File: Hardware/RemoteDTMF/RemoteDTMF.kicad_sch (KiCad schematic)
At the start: 35 parts, among them J1 REG. 7V, J10 MT8870D, J11 P12V, J2 BATT 12V, J3 P12V, J4 Analog, J5 Digital, J6 TRX TELCO, J7 AL. ATTINY85, J8 IO ATTINY85, J9 AT-D578, U1 PC817, U2 PC817, U3 CD4066BE, U4 PC817

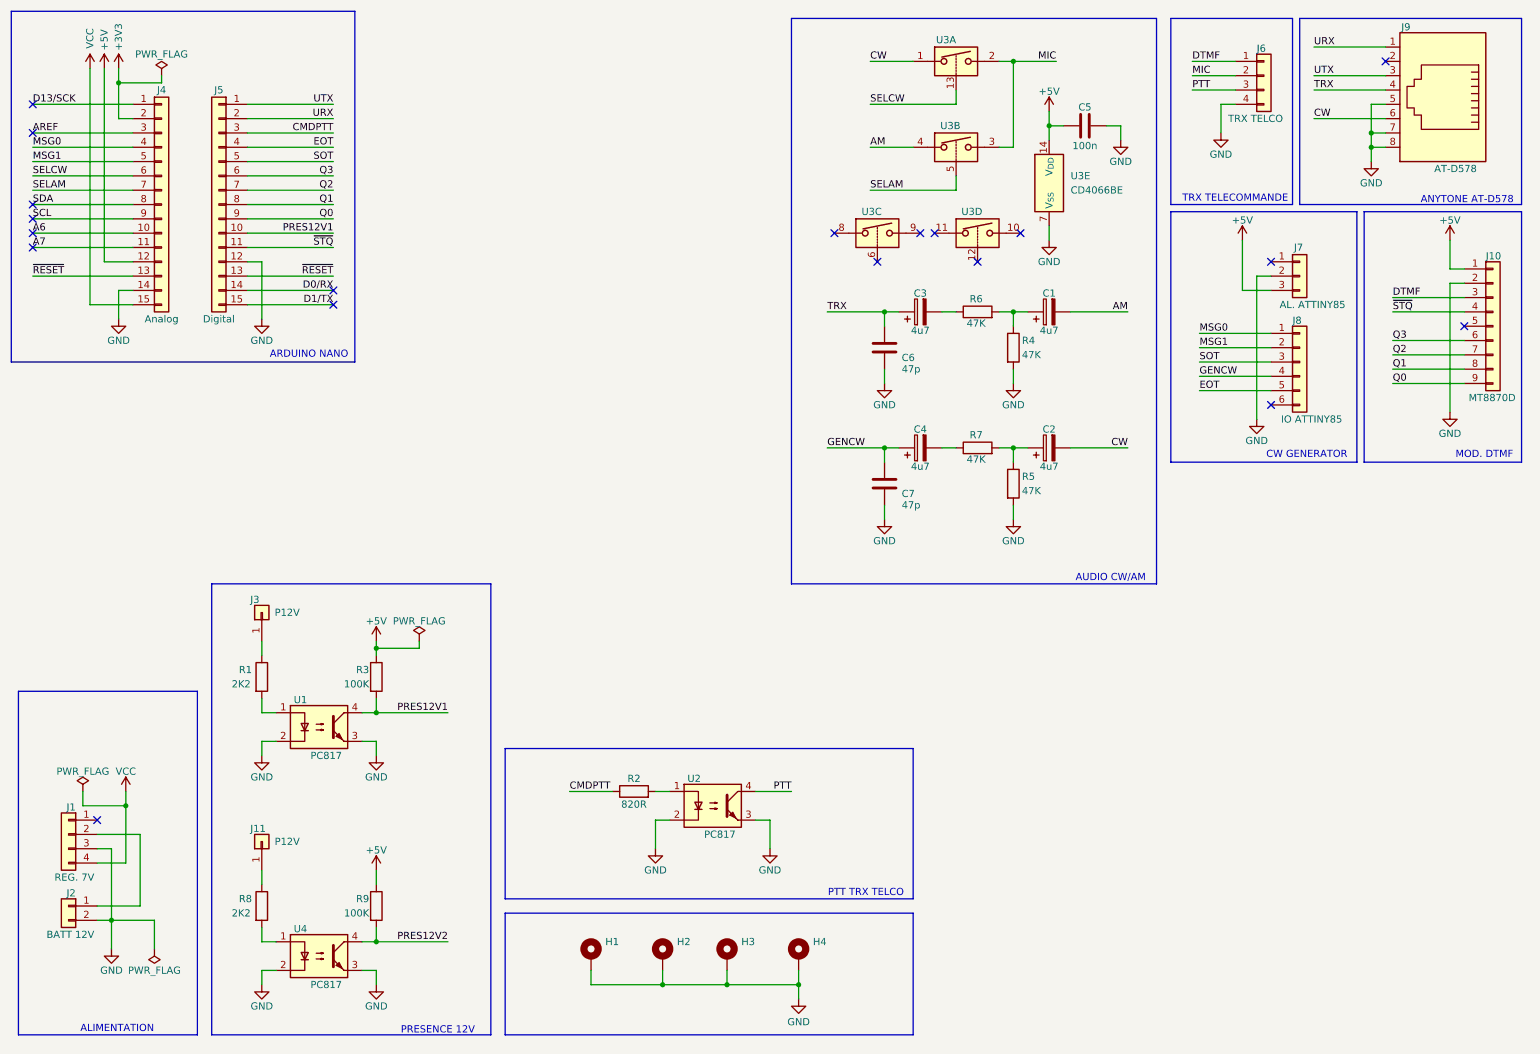
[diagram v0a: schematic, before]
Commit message: Update Schematic & WIP 0.6A
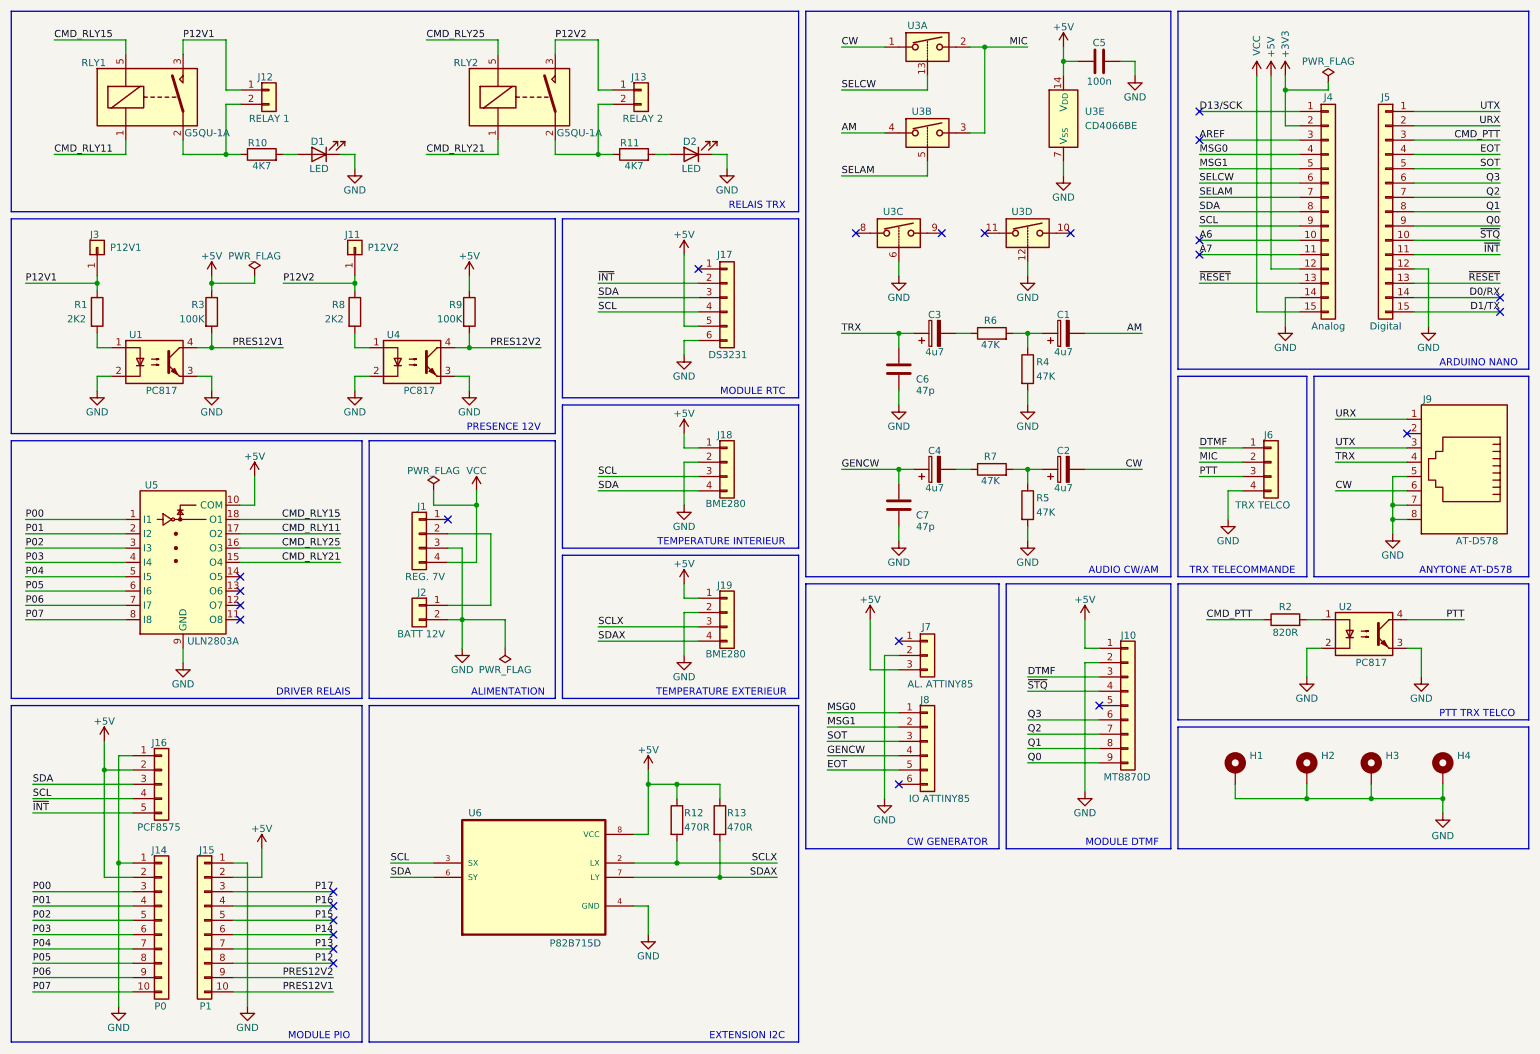
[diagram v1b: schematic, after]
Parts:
- added D1, D2: LED, LED_THT:LED_D3.0mm, symbol Device:LED
- added J12: RELAY 1, TerminalBlock:TerminalBlock_MaiXu_MX126-5.0-02P_1x02_P5.00mm, symbol Connector_Generic:Conn_01x02
- added J13: RELAY 2, TerminalBlock:TerminalBlock_MaiXu_MX126-5.0-02P_1x02_P5.00mm, symbol Connector_Generic:Conn_01x02
- added J14: P0, Connector_PinHeader_2.54mm:PinHeader_1x10_P2.54mm_Vertical, symbol Connector_Generic:Conn_01x10
- added J15: P1, Connector_PinHeader_2.54mm:PinHeader_1x10_P2.54mm_Vertical, symbol Connector_Generic:Conn_01x10
- added J16: PCF8575, Connector_PinHeader_2.54mm:PinHeader_1x05_P2.54mm_Vertical, symbol Connector_Generic:Conn_01x05
- added J17: DS3231, Connector_PinHeader_2.54mm:PinHeader_1x06_P2.54mm_Vertical, symbol Connector_Generic:Conn_01x06
- added J18, J19: BME280, Connector_PinHeader_2.54mm:PinHeader_1x04_P2.54mm_Vertical, symbol Connector_Generic:Conn_01x04
- added R10, R11: 4K7, Resistor_THT:R_Axial_DIN0204_L3.6mm_D1.6mm_P7.62mm_Horizontal, symbol Device:R
- added R12, R13: 470R, Resistor_THT:R_Axial_DIN0204_L3.6mm_D1.6mm_P7.62mm_Horizontal, symbol Device:R
- added RLY1, RLY2: G5QU-1A, Relay_THT:Relay_SPST_Omron-G5Q-1A, symbol Relay:G5Q-1A
- added U5: ULN2803A, Package_DIP:DIP-18_W7.62mm, symbol Transistor_Array:ULN2803A
- added U6: P82B715D, Package_DIP:DIP-8_W7.62mm, symbol P82B715D:P82B715D
- J11: value P12V -> P12V2
- J3: value P12V -> P12V1
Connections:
- net +5V: now also J14.2 (Pin_2), J15.2 (Pin_2), J16.2 (Pin_2), J17.5 (Pin_5), J18.1 (Pin_1), J19.1 (Pin_1), R12.1, R13.1, U5.10 (COM), U6.8 (VCC)
- net GND: now also U3.12, U3.6, D1.1 (K), D2.1 (K), J14.1 (Pin_1), J15.1 (Pin_1), J16.1 (Pin_1), J17.6 (Pin_6), J18.2 (Pin_2), J19.2 (Pin_2), U5.9 (GND), U6.4 (GND)
- net PRES12V1: now also J15.10 (Pin_10); no longer J5.10 (Pin_10)
- net PRES12V2: now also J15.9 (Pin_9)
- net SCL: now also J16.4 (Pin_4), J17.4 (Pin_4), J18.3 (Pin_3), U6.3 (SX)
- net SDA: now also J16.3 (Pin_3), J17.3 (Pin_3), J18.4 (Pin_4), U6.6 (SY)
- net ~{STQ}: now also J5.10 (Pin_10); no longer J5.11 (Pin_11)
- net P12V2: now reaches J11.1 (Pin_1), R8.1
- net P12V2: now also J13.1 (Pin_1), RLY2.3
- net P12V1: now reaches J3.1 (Pin_1), R1.1
- net P12V1: now also J12.1 (Pin_1), RLY1.3
- net CMDPTT renamed CMD_PTT
- new net: J13.2 (Pin_2), R11.1, RLY2.2
- new net: D1.2 (A), R10.2
- new net: J12.2 (Pin_2), R10.1, RLY1.2
- new net: D2.2 (A), R11.2
- new net CMD_RLY11: RLY1.1, U5.17 (O2)
- new net CMD_RLY15: RLY1.5, U5.18 (O1)
- new net CMD_RLY21: RLY2.1, U5.15 (O4)
- new net CMD_RLY25: RLY2.5, U5.16 (O3)
- new net P00: J14.3 (Pin_3), U5.1 (I1)
- new net P01: J14.4 (Pin_4), U5.2 (I2)
- new net P02: J14.5 (Pin_5), U5.3 (I3)
- new net P03: J14.6 (Pin_6), U5.4 (I4)
- new net P04: J14.7 (Pin_7), U5.5 (I5)
- new net P05: J14.8 (Pin_8), U5.6 (I6)
- new net P06: J14.9 (Pin_9), U5.7 (I7)
- new net P07: J14.10 (Pin_10), U5.8 (I8)
- new net P12: J15.8 (Pin_8)
- new net P13: J15.7 (Pin_7)
- new net P14: J15.6 (Pin_6)
- new net P15: J15.5 (Pin_5)
- new net P16: J15.4 (Pin_4)
- new net P17: J15.3 (Pin_3)
- new net SCLX: J19.3 (Pin_3), R12.2, U6.2 (LX)
- new net SDAX: J19.4 (Pin_4), R13.2, U6.7 (LY)
- new net ~{INT}: J16.5 (Pin_5), J17.2 (Pin_2), J5.11 (Pin_11)
- no-connect marks 19 -> 26
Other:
- note added: "DRIVER RELAIS"
- note added: "EXTENSION I2C"
- note added: "MODULE DTMF"
- note added: "MODULE PIO"
- note added: "MODULE RTC"
- note added: "RELAIS TRX"
- note added: "TEMPERATURE EXTERIEUR"
- note added: "TEMPERATURE INTERIEUR"
- note removed: "MOD. DTMF"
- moved on the sheet: C1, C2, C3, C4, C5, C6, C7, H1, H2, H3, H4, J1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
